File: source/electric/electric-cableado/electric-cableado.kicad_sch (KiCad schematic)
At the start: 100 parts

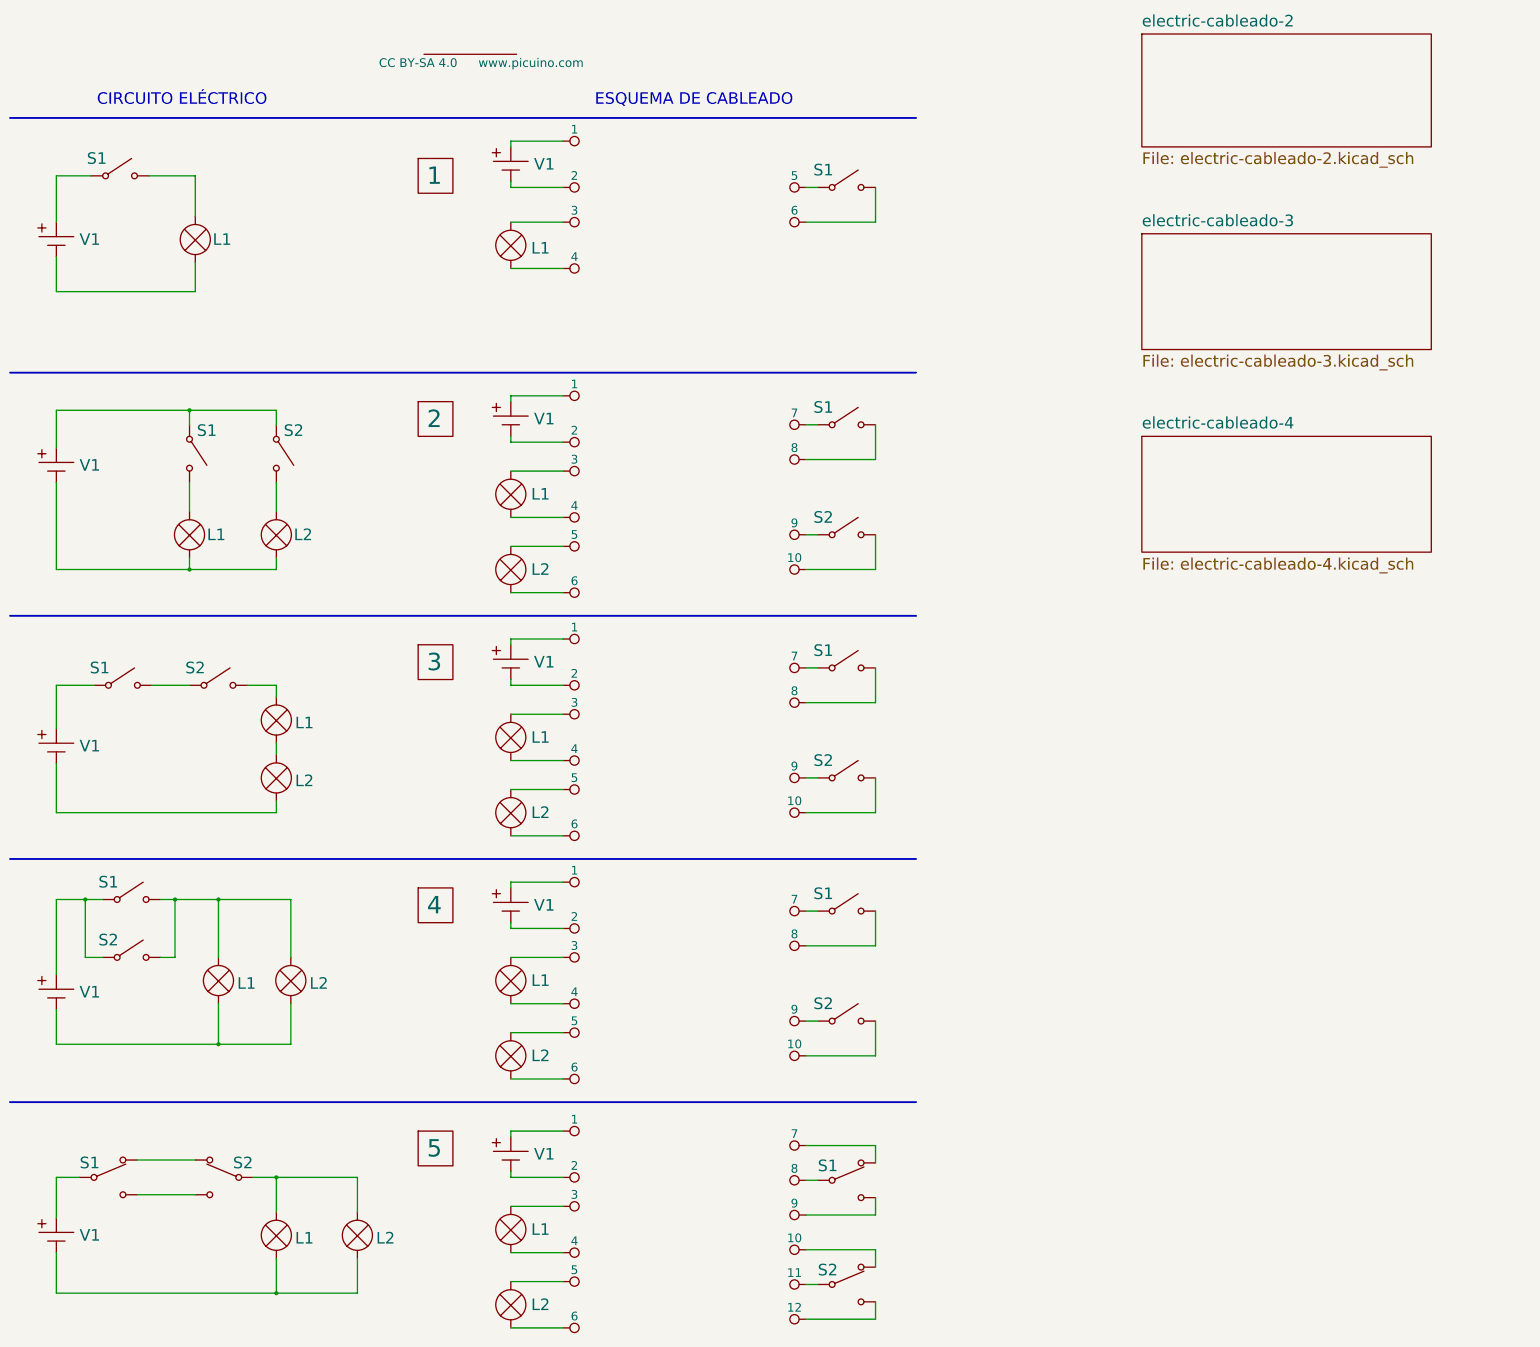
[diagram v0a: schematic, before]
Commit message: 25/01/2025 Update
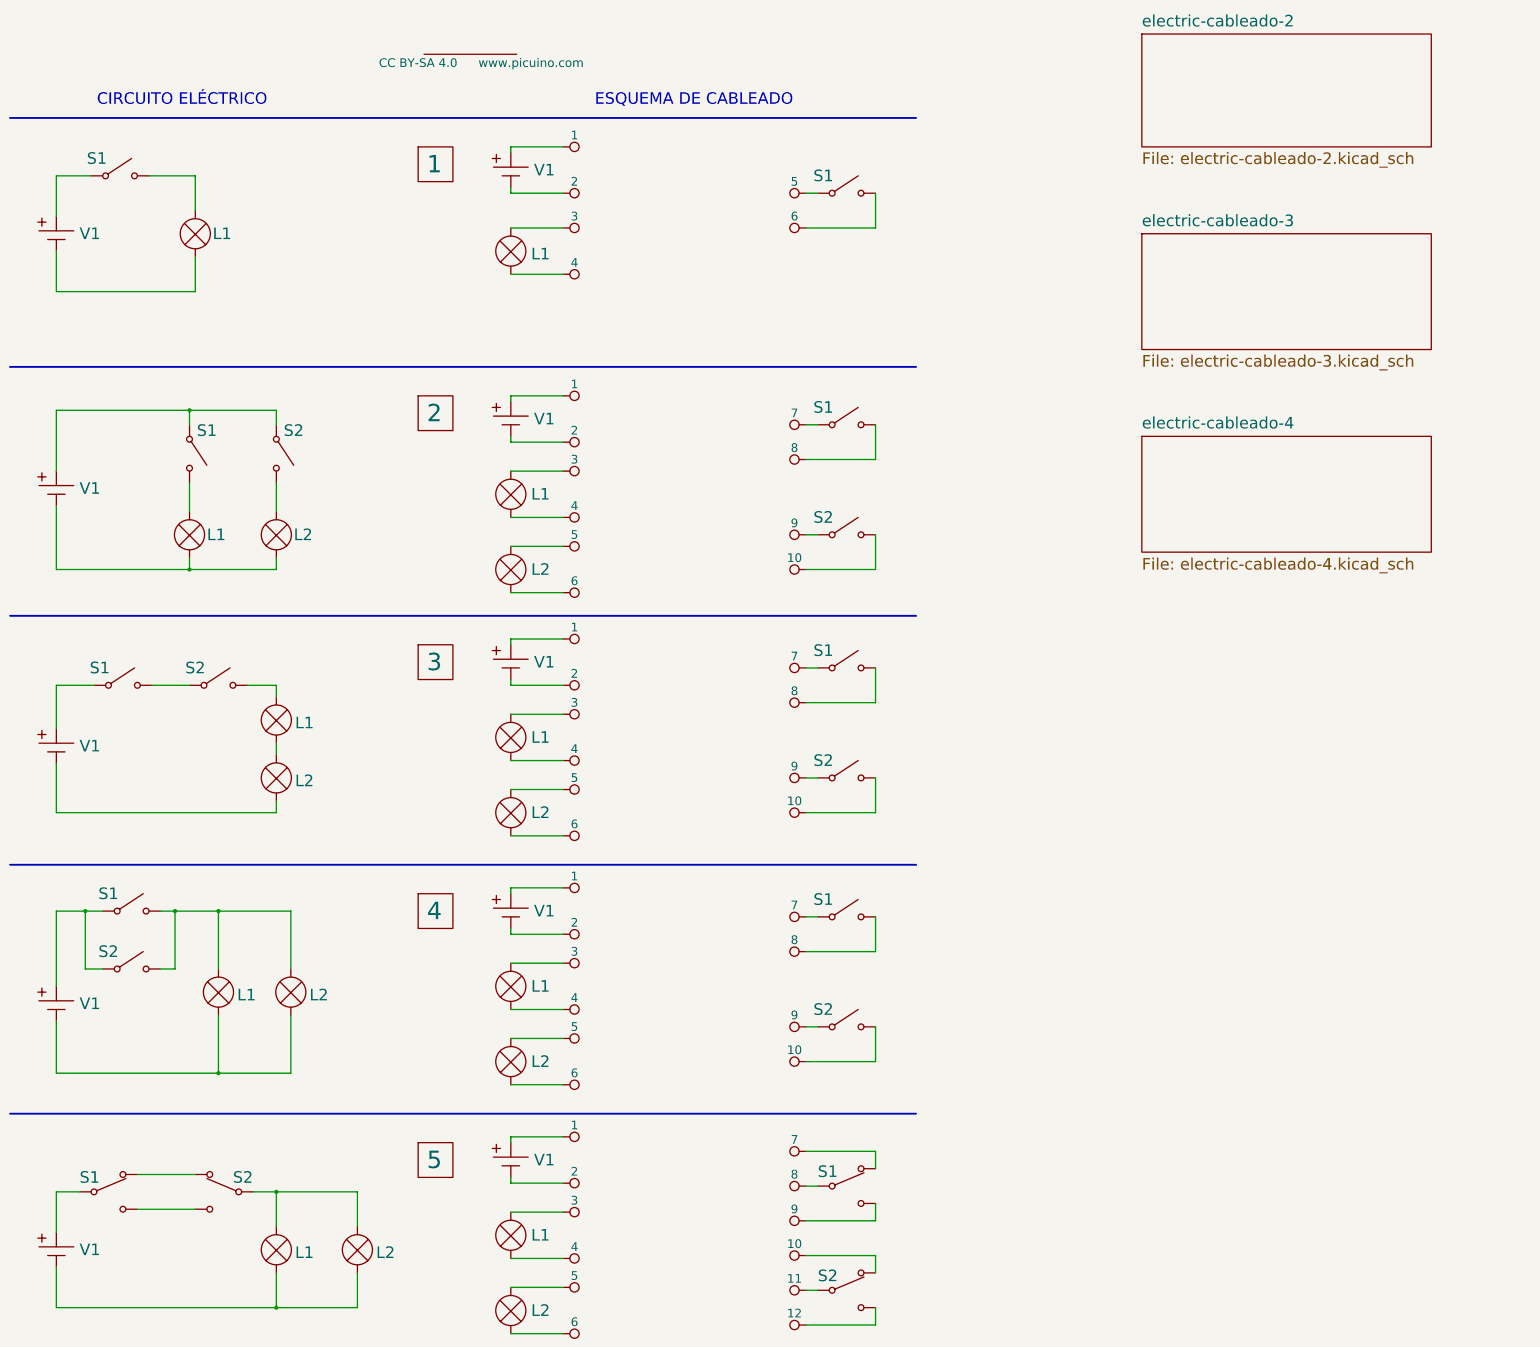
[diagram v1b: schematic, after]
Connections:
- net at S1.: now also L1.; no longer V1.
- net at L1.: now also V1.; no longer S1.
- net at V1.: now also S1.; no longer L2.
- net at S1.: now also S2.; no longer V1.
- net at S1., S2.: now also L1., L2.; no longer V1.
- net at V1.: now also L1., L2.; no longer S1.
- net at L1., L2.: now also S2.; no longer V1.
- new net: S1., V1. (x2)
- new net: L2., V1.
- new net: S1., S2., V1. (x2)
- new net: L1., L2., V1.
- new net: S1., S2.
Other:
- moved on the sheet: L1, L2, S1, S2, V1
